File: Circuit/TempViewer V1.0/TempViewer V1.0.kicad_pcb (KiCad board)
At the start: 2 copper layers, 121 parts, among them J1 Screw_Terminal_01x02, J10 InterLock_3, J11 InterLock_4, J2 12V IN, J3 Programming, J4 12V OUT, J5 5V IN, J6 I2C, J7 5V OUT, J8 InterLock_1, J9 InterLock_2, K1 EE2-5NU, K2 EE2-5NU, K3 EE2-5NU, K4 EE2-5NU, Q1 DMN3731U, Q10 DMN3731U, Q2 DMN3731U, Q3 DMN3731U, Q4 DMN3731U, Q5 DMN3731U, Q6 DMN3731U, Q7 DMN3731U, Q8 DMN3731U, Q9 DMN3731U, U1 LTC2451xDDB, U10 ATA00AA36S-L, U11 TLV1117-33, U13 LTC1798CS8-3PBF, U14 LM7805_TO220, U2 PIC16F18877-I/PT, U4 MAX4289ESA+ / OP37, U5 MAX4289ESA+ / OP37, U6 ISO1641BDR, U7 AD5272BCP, U8 AD5272BCP, U9 TLP2770

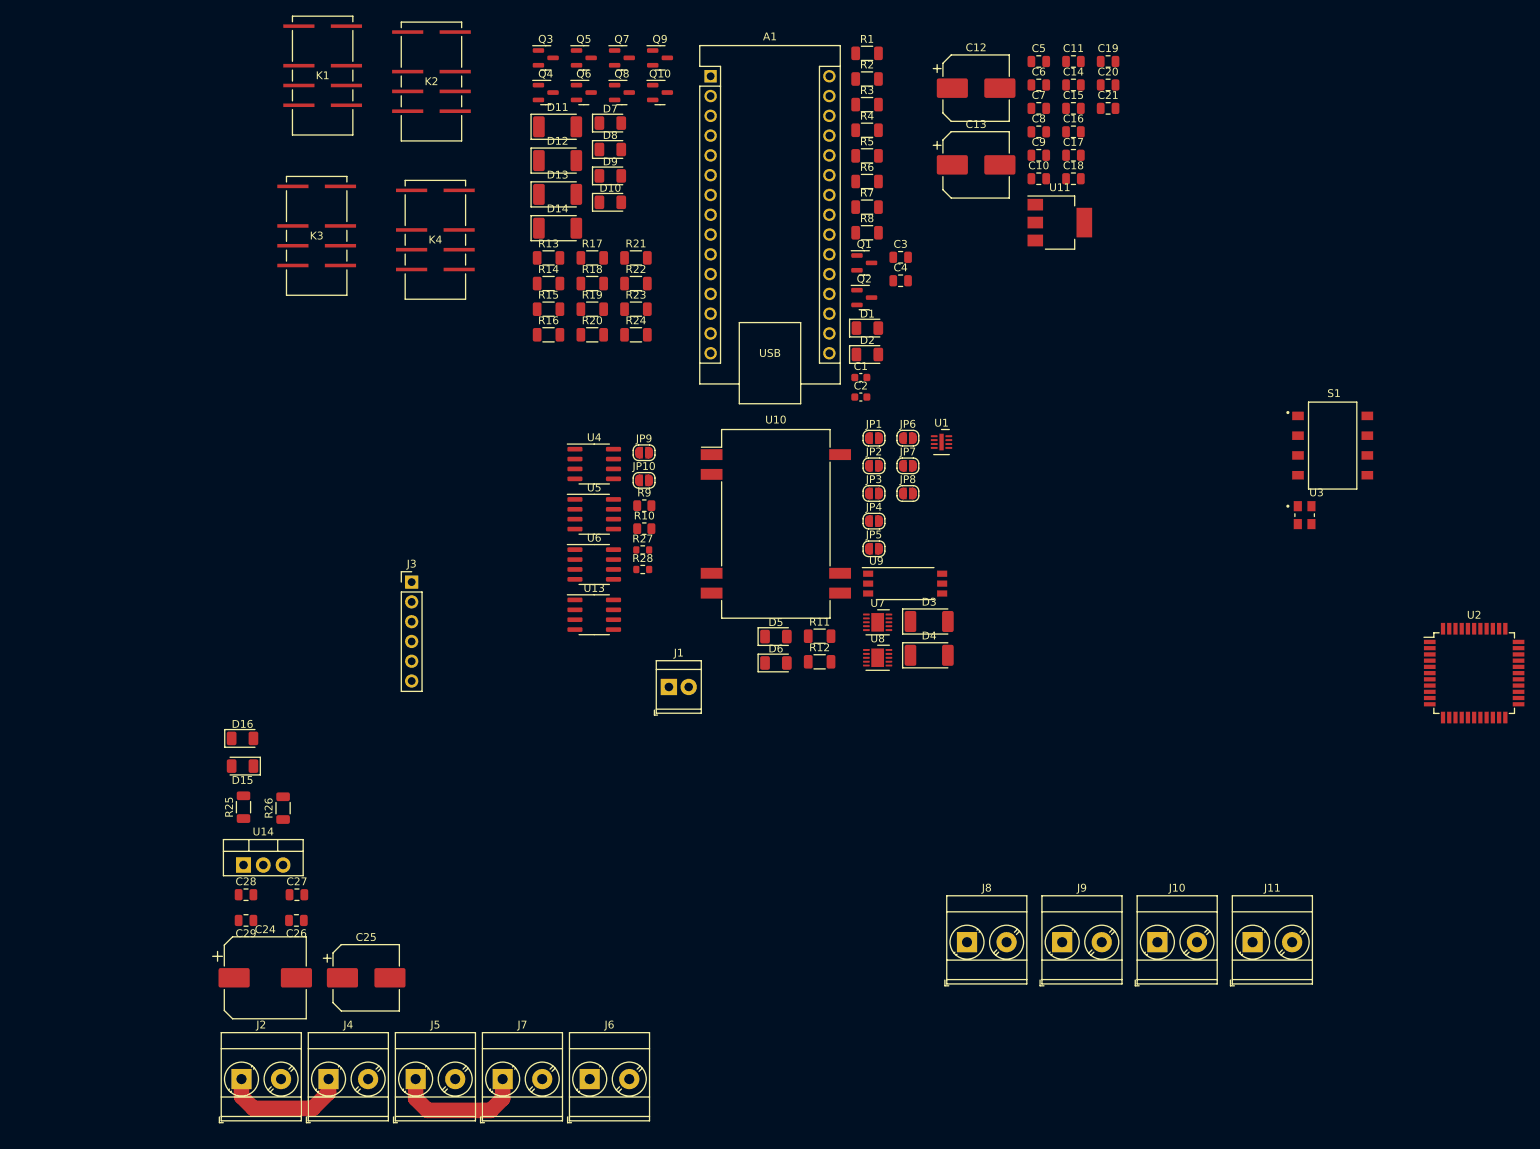
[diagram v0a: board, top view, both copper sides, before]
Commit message: PCB Design V1
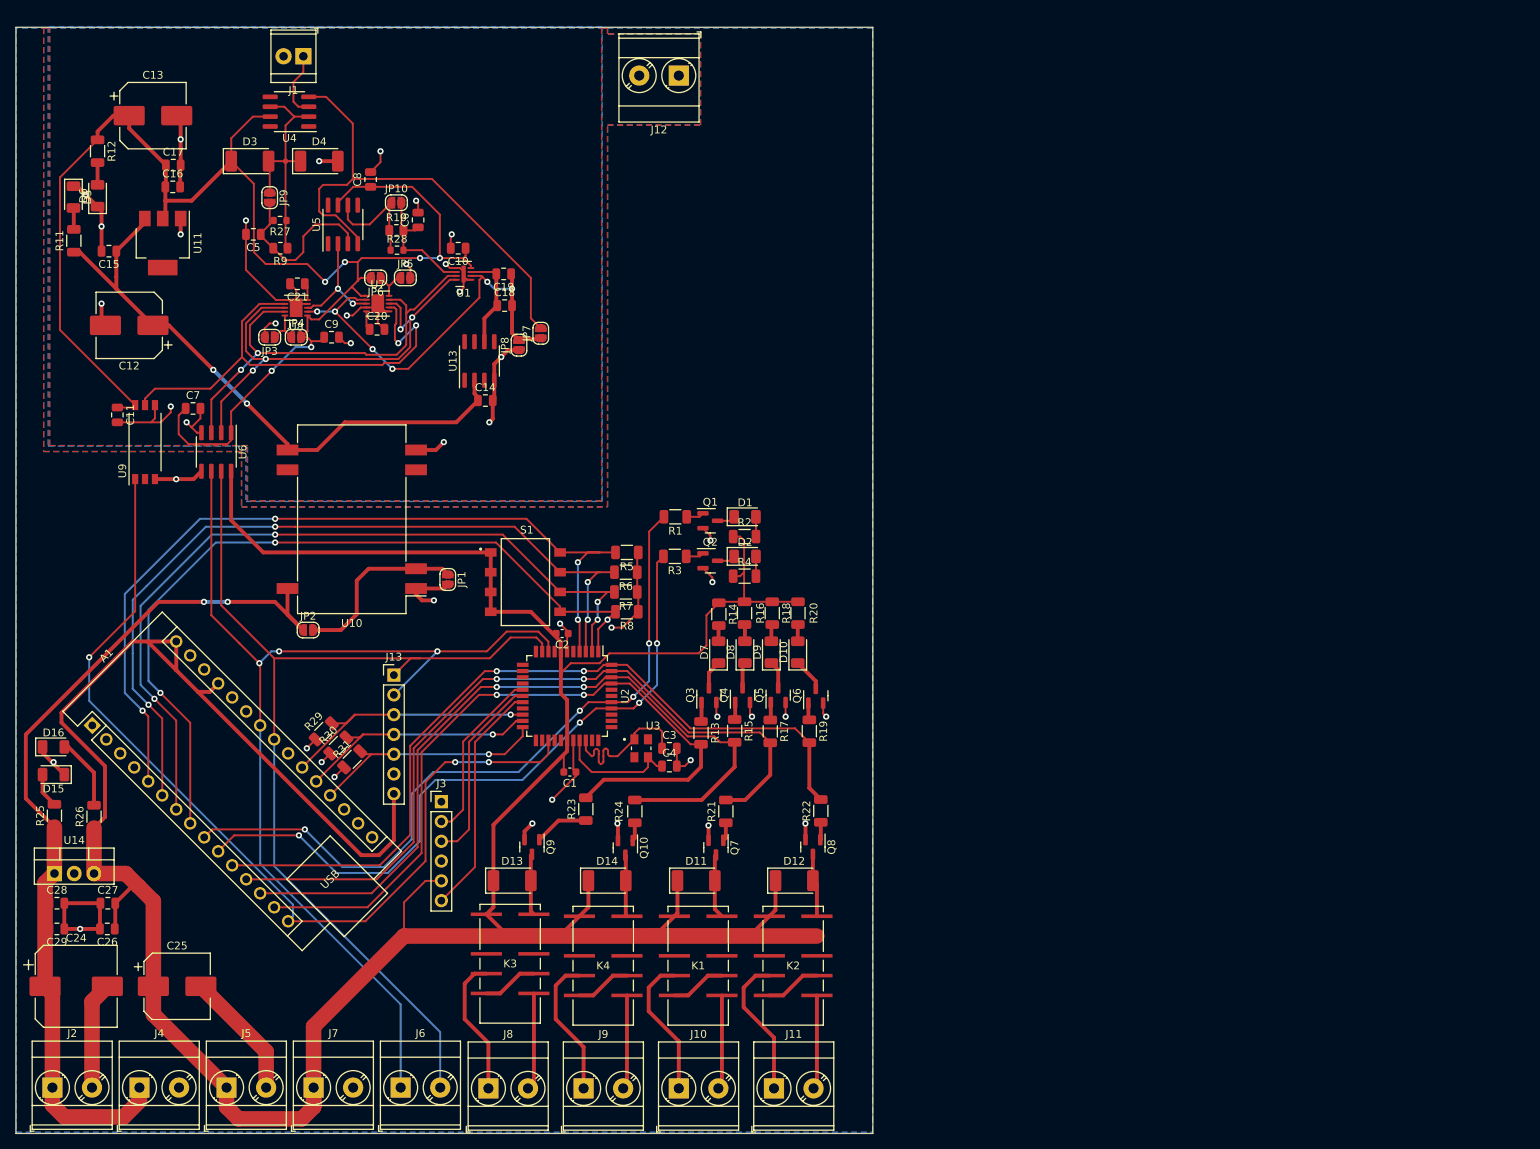
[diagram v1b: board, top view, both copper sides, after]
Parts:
- added J12: PE, TerminalBlock_Phoenix:TerminalBlock_Phoenix_MKDS-3-2-5.08_1x02_P5.08mm_Horizontal, F.Cu at (85.1, 44.2)
- added J13: Conn_01x07_Pin, Connector_PinHeader_2.54mm:PinHeader_1x07_P2.54mm_Vertical, F.Cu at (48.5, 121.2)
- added R29: 10KR, Resistor_SMD:R_1206_3216Metric, F.Cu at (39.5, 128.4)
- added R30: 10KR, Resistor_SMD:R_1206_3216Metric, F.Cu at (41.4, 130.2)
- added R31: 10KR, Resistor_SMD:R_1206_3216Metric, F.Cu at (43.2, 132.0)
- moved C11 130.9 mm to (13.0, 87.8), turned to -90 degrees
- moved C15 125.2 mm to (11.9, 66.7), turned to 180 degrees
- moved K1 124.0 mm to (87.6, 158.5)
- moved K2 122.6 mm to (99.8, 158.5)
- moved U2 116.5 mm to (70.8, 123.8), turned to -90 degrees
- moved C16 115.8 mm to (20.1, 58.5)
- moved C17 115.6 mm to (20.2, 55.7)
- moved C7 115.2 mm to (22.7, 86.9)
- moved U11 115.2 mm to (18.8, 65.7), turned to -90 degrees
- moved A1 115.1 mm to (9.80, 127.6), turned to 45 degrees
- moved R12 113.5 mm to (10.5, 53.9), turned to -90 degrees
- moved C12 112.9 mm to (14.5, 76.3), turned to 180 degrees
- moved R11 108.4 mm to (7.43, 65.4), turned to 90 degrees
- moved C21 106.5 mm to (36.1, 70.9), turned to 180 degrees
- moved D5 106.4 mm to (7.38, 59.8), turned to -90 degrees
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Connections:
- A1 pad 10: ADDR_1 -> ERRLED
- A1 pad 11: Interlock_1 -> Interlock_4
- A1 pad 12: Interlock_2 -> Interlock_3
- A1 pad 14: Interlock_2 -> Interlock_1
- A1 pad 15: unconnected-(A1-D12-Pad15) -> ResetR
- A1 pad 5: CycleLED -> ADDR_1
- A1 pad 6: ERRLED -> ADDR_2
- A1 pad 7: ADDR_4 -> ADDR_3
- A1 pad 8: ADDR_3 -> ADDR_4
- A1 pad 9: ADDR_2 -> CycleLED
- U2 pad 25: unconnected-(U2-RE0-Pad25) -> ResetR
- U5 pad 4: A3V3 -> -VREF
- U5 pad 7: VREF -> A3V3
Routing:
- net 5V: track 17.4 -> 459.2 mm
- net A3V3: track 0.00 -> 201.8 mm, vias 0 -> 6
- net SCL: track 0.00 -> 137.7 mm, vias 0 -> 3
- net SDA: track 0.00 -> 131.8 mm
- net ResetR: track 0.00 -> 120.6 mm, vias 0 -> 3
- net GND: track 0.00 -> 120.1 mm, vias 0 -> 21
- net AGND: track 0.00 -> 109.2 mm, vias 0 -> 21
- net ADDR_1: track 0.00 -> 109.0 mm, vias 0 -> 4
- net ADDR_2: track 0.00 -> 105.9 mm, vias 0 -> 4
- net ADDR_3: track 0.00 -> 104.2 mm, vias 0 -> 4
- net Interlock_4: track 0.00 -> 103.5 mm, vias 0 -> 2
- net ADDR_4: track 0.00 -> 103.2 mm, vias 0 -> 3
- net Interlock_2: track 0.00 -> 100.9 mm, vias 0 -> 2
- net Interlock_3: track 0.00 -> 100.4 mm, vias 0 -> 2
- net 12V: track 16.6 -> 114.7 mm, vias 0 -> 2
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- added copper zone on B.Cu, net AGND
- added copper zone on B.Cu, net GND
- added copper zone on B.Cu, net PE
- added copper zone on F.Cu, net PE
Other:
- board outline added: 110 x 142 mm
